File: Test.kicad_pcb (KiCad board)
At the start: 4 copper layers, 111.8 x 100.3 mm, 41 parts, among them P1 CONN_01X12, P10 CONN_01X12, P10a1 CONN_01X10, P11 CONN_01X03, P12 CONN_01X04, P13 CONN_02X04, P14 CONN_02X03, P15 CONN_02X05, P16 CONN_01X05, P17 CONN_01X01, P18 CONN_01X02, P19 CONN_01X08, P1a1 CONN_01X10, P2 CONN_01X12, P20 CONN_01X05, P21 CONN_01X05, P22 CONN_01X04, P23 CONN_01X04, P24 CONN_01X03, P25 CONN_01X10, P26 CONN_01X10, P27 CONN_01X10, P28 CONN_01X10, P2a1 CONN_01X10, P2a2 CONN_01X03, P2a3 CONN_01X03, P3 CONN_01X03, P4 CONN_01X24, P5 CONN_01X24, P6 CONN_01X03, P7 CONN_01X24, P8 CONN_01X24, P9 CONN_01X12, P9a1 CONN_01X10, SW1 SW_PUSH_SMALL_H, SW2 SW_PUSH_SMALL_H

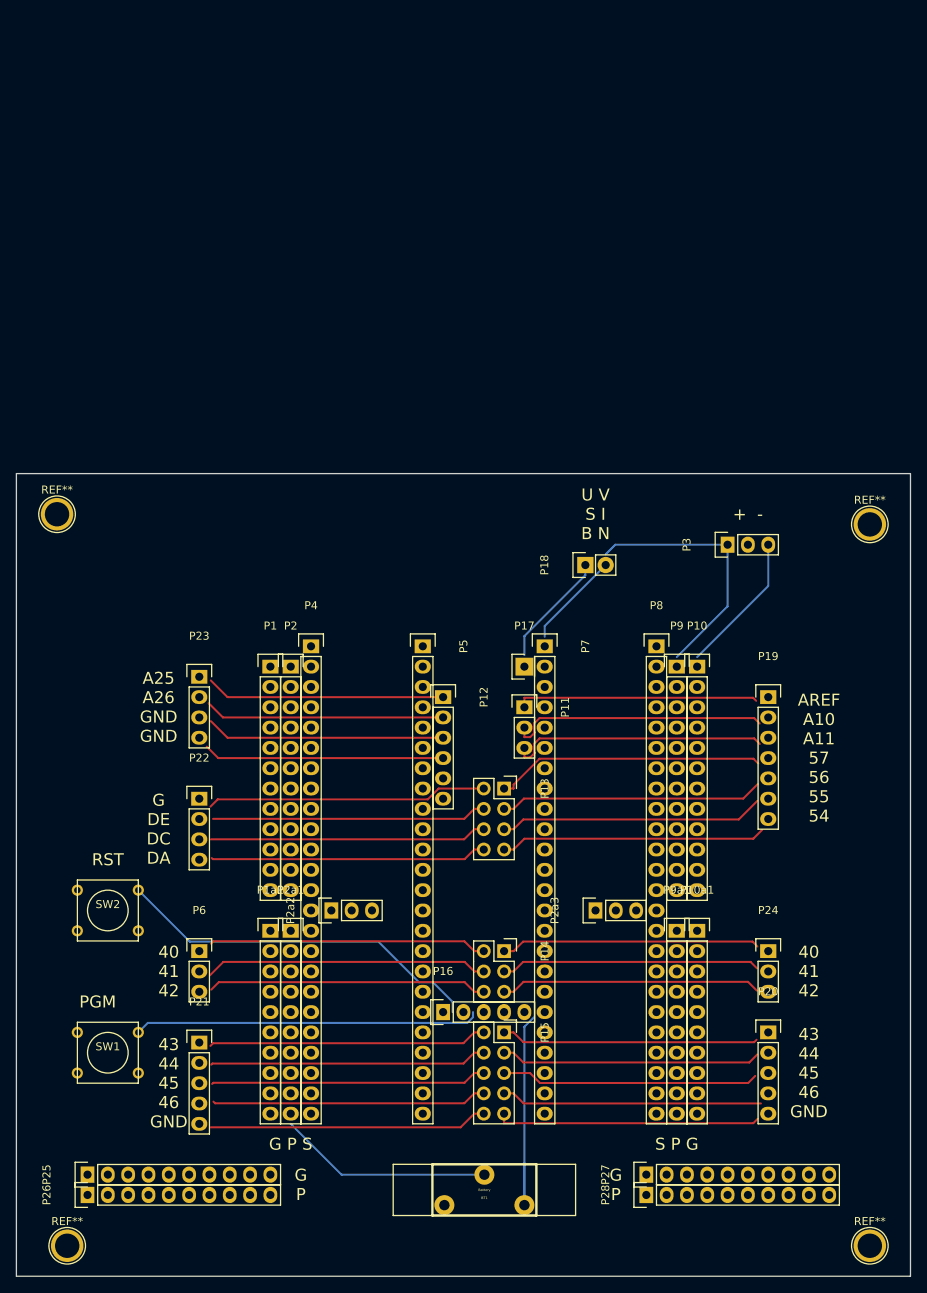
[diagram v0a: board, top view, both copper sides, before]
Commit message: Version 2
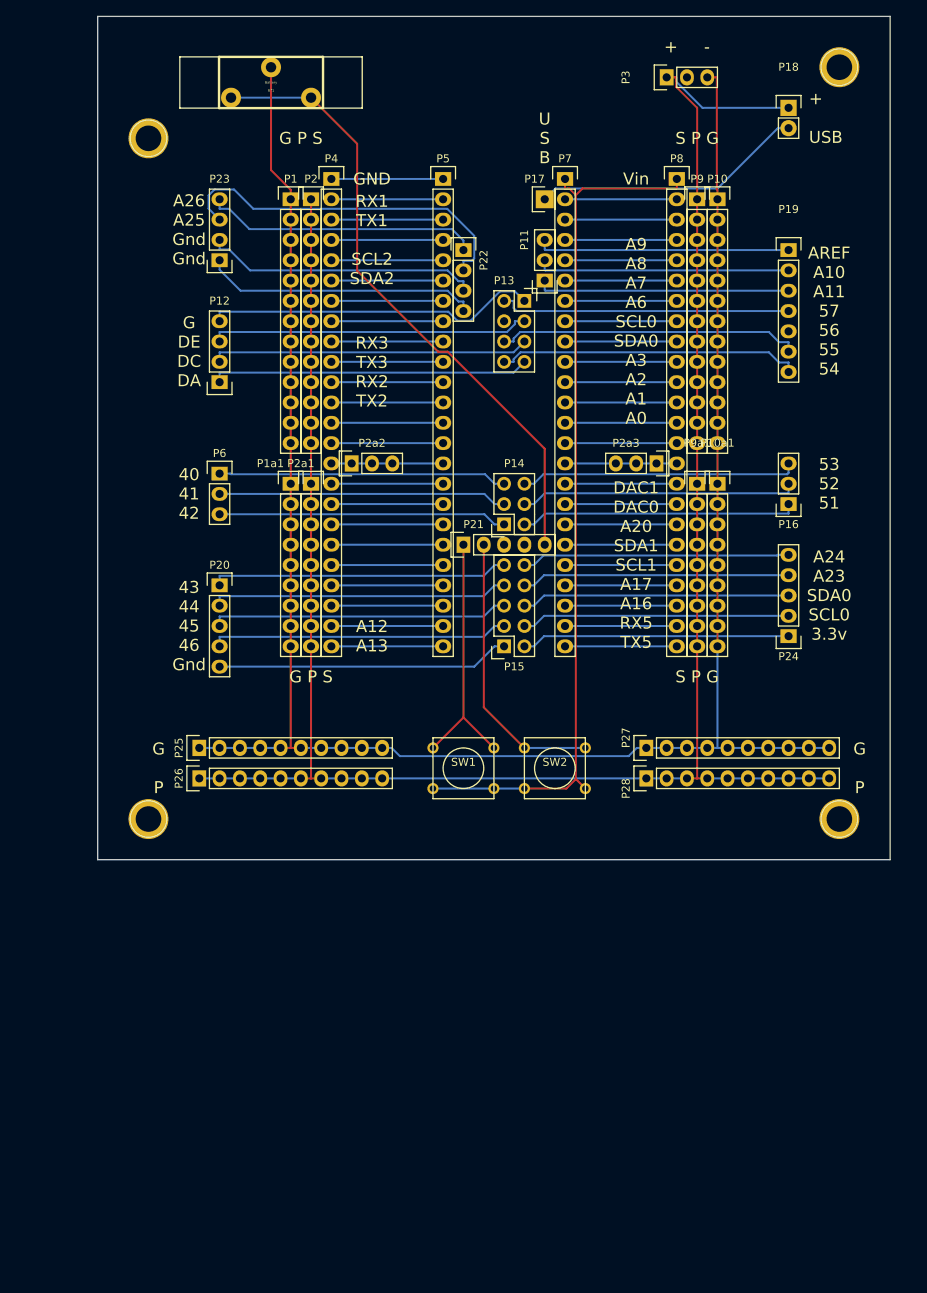
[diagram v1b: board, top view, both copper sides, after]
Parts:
- removed the REF** at (57.1, 184.2)
- removed the REF** at (157.5, 184.2)
- removed the REF** at (157.5, 94.0)
- removed the REF** at (55.9, 92.7)
- added REF**: 1pin, Connect:1pin, F.Cu at (153.7, 36.8)
- added REF**: 1pin, Connect:1pin, F.Cu at (67.3, 45.7)
- added REF**: 1pin, Connect:1pin, F.Cu at (67.3, 130.8)
- added REF**: 1pin, Connect:1pin, F.Cu at (153.7, 130.8)
- P1, P10, P2, P9: value CONN_01X12 -> CONN_01X13; footprint Pin_Headers:Pin_Header_Straight_1x12 -> Pin_Headers:Pin_Header_Straight_1x13
- P10a1: footprint Pin_Headers:Pin_Header_Straight_1x10 -> Pin_Headers:Pin_Header_Straight_1x09
- P12: footprint Socket_Strips:Socket_Strip_Straight_1x06 -> Pin_Headers:Pin_Header_Straight_1x04
- P16: value CONN_01X05 -> CONN_01X03; footprint Socket_Strips:Socket_Strip_Straight_1x05 -> Pin_Headers:Pin_Header_Straight_1x03
- P1a1, P2a1, P9a1: value CONN_01X10 -> CONN_01X09; footprint Pin_Headers:Pin_Header_Straight_1x10 -> Pin_Headers:Pin_Header_Straight_1x09
- P21: footprint Pin_Headers:Pin_Header_Straight_1x05 -> Socket_Strips:Socket_Strip_Straight_1x05
- P22: footprint Pin_Headers:Pin_Header_Straight_1x04 -> Socket_Strips:Socket_Strip_Straight_1x04
- P24: value CONN_01X03 -> CONN_01X05; footprint Pin_Headers:Pin_Header_Straight_1x03 -> Pin_Headers:Pin_Header_Straight_1x05
- moved BT1 141.0 mm to (82.6, 38.7)
- moved P20 88.5 mm to (76.2, 101.6)
- moved P16 76.8 mm to (147.3, 91.4), turned to 180 degrees
- moved P22 76.1 mm to (106.7, 59.7), turned to 270 degrees
- moved P21 70.4 mm to (106.7, 96.5)
- moved P18 62.5 mm to (147.3, 41.9), turned to 0 degrees
- moved P13 61.0 mm to (114.3, 66.0)
- moved P6 59.7 mm to (76.2, 87.6)
- moved P3 58.9 mm to (132.1, 38.1)
- moved SW2 58.6 mm to (118.1, 124.5)
- moved P1 58.5 mm to (85.1, 53.3)
- moved P10 58.5 mm to (138.4, 53.3)
- moved P17 58.5 mm to (116.8, 53.3)
- moved P2 58.5 mm to (87.6, 53.3)
- moved P4 58.5 mm to (90.2, 50.8)
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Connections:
- P1 pad 1: Net-(P1-Pad1) -> Net-(BT1-Pad2)
- P1 pad 10: Net-(P1-Pad1) -> Net-(BT1-Pad2)
- P1 pad 11: Net-(P1-Pad1) -> Net-(BT1-Pad2)
- P1 pad 12: Net-(P1-Pad1) -> Net-(BT1-Pad2)
- P1 pad 2: Net-(P1-Pad1) -> Net-(BT1-Pad2)
- P1 pad 3: Net-(P1-Pad1) -> Net-(BT1-Pad2)
- P1 pad 4: Net-(P1-Pad1) -> Net-(BT1-Pad2)
- P1 pad 5: Net-(P1-Pad1) -> Net-(BT1-Pad2)
- P1 pad 6: Net-(P1-Pad1) -> Net-(BT1-Pad2)
- P1 pad 7: Net-(P1-Pad1) -> Net-(BT1-Pad2)
- P1 pad 8: Net-(P1-Pad1) -> Net-(BT1-Pad2)
- P1 pad 9: Net-(P1-Pad1) -> Net-(BT1-Pad2)
- P10 pad 1: Net-(P10-Pad1) -> Net-(BT1-Pad2)
- P10 pad 10: Net-(P10-Pad1) -> Net-(BT1-Pad2)
- P10 pad 11: Net-(P10-Pad1) -> Net-(BT1-Pad2)
- P10 pad 12: Net-(P10-Pad1) -> Net-(BT1-Pad2)
- P10 pad 2: Net-(P10-Pad1) -> Net-(BT1-Pad2)
- P10 pad 3: Net-(P10-Pad1) -> Net-(BT1-Pad2)
- P10 pad 4: Net-(P10-Pad1) -> Net-(BT1-Pad2)
- P10 pad 5: Net-(P10-Pad1) -> Net-(BT1-Pad2)
- P10 pad 6: Net-(P10-Pad1) -> Net-(BT1-Pad2)
- P10 pad 7: Net-(P10-Pad1) -> Net-(BT1-Pad2)
- P10 pad 8: Net-(P10-Pad1) -> Net-(BT1-Pad2)
- P10 pad 9: Net-(P10-Pad1) -> Net-(BT1-Pad2)
- P10a1 pad 1: Net-(P10a1-Pad1) -> Net-(BT1-Pad2)
- P10a1 pad 2: Net-(P10a1-Pad1) -> Net-(BT1-Pad2)
- P10a1 pad 3: Net-(P10a1-Pad1) -> Net-(BT1-Pad2)
- P10a1 pad 4: Net-(P10a1-Pad1) -> Net-(BT1-Pad2)
- P10a1 pad 5: Net-(P10a1-Pad1) -> Net-(BT1-Pad2)
- P10a1 pad 6: Net-(P10a1-Pad1) -> Net-(BT1-Pad2)
- P10a1 pad 7: Net-(P10a1-Pad1) -> Net-(BT1-Pad2)
- P10a1 pad 8: Net-(P10a1-Pad1) -> Net-(BT1-Pad2)
- P10a1 pad 9: Net-(P10a1-Pad1) -> Net-(BT1-Pad2)
- P13 pad 1: Net-(P13-Pad1) -> Net-(P12-Pad4)
- P13 pad 3: Net-(P13-Pad3) -> Net-(P12-Pad3)
- P13 pad 5: Net-(P13-Pad5) -> Net-(P12-Pad2)
- P13 pad 7: Net-(P13-Pad7) -> Net-(P12-Pad1)
- P16 pad 1: Net-(P16-Pad1) -> Net-(P14-Pad2)
- P16 pad 2: Net-(P16-Pad2) -> Net-(P14-Pad4)
- P16 pad 3: Net-(P16-Pad3) -> Net-(P14-Pad6)
- P18 pad 2: Net-(P18-Pad2) -> Net-(P17-Pad1)
- P19 pad 1: Net-(P19-Pad1) -> Net-(P11-Pad3)
- P19 pad 2: Net-(P19-Pad2) -> Net-(P11-Pad2)
- P19 pad 3: Net-(P19-Pad3) -> Net-(P11-Pad1)
- P19 pad 4: Net-(P19-Pad4) -> Net-(P13-Pad2)
- P19 pad 6: Net-(P19-Pad6) -> Net-(P13-Pad6)
- P19 pad 7: Net-(P19-Pad7) -> Net-(P13-Pad8)
- P1a1 pad 1: Net-(P1a1-Pad1) -> Net-(BT1-Pad2)
- P1a1 pad 2: Net-(P1a1-Pad1) -> Net-(BT1-Pad2)
- P1a1 pad 3: Net-(P1a1-Pad1) -> Net-(BT1-Pad2)
- P1a1 pad 4: Net-(P1a1-Pad1) -> Net-(BT1-Pad2)
- P1a1 pad 5: Net-(P1a1-Pad1) -> Net-(BT1-Pad2)
- P1a1 pad 6: Net-(P1a1-Pad1) -> Net-(BT1-Pad2)
- P1a1 pad 7: Net-(P1a1-Pad1) -> Net-(BT1-Pad2)
- P1a1 pad 8: Net-(P1a1-Pad1) -> Net-(BT1-Pad2)
- P1a1 pad 9: Net-(P1a1-Pad1) -> Net-(BT1-Pad2)
- P2 pad 1: Net-(P2-Pad1) -> Net-(P18-Pad1)
- P2 pad 10: Net-(P2-Pad1) -> Net-(P18-Pad1)
- P2 pad 11: Net-(P2-Pad1) -> Net-(P18-Pad1)
- P2 pad 12: Net-(P2-Pad1) -> Net-(P18-Pad1)
- P2 pad 2: Net-(P2-Pad1) -> Net-(P18-Pad1)
- P2 pad 3: Net-(P2-Pad1) -> Net-(P18-Pad1)
- P2 pad 4: Net-(P2-Pad1) -> Net-(P18-Pad1)
- P2 pad 5: Net-(P2-Pad1) -> Net-(P18-Pad1)
- P2 pad 6: Net-(P2-Pad1) -> Net-(P18-Pad1)
- P2 pad 7: Net-(P2-Pad1) -> Net-(P18-Pad1)
- P2 pad 8: Net-(P2-Pad1) -> Net-(P18-Pad1)
- P2 pad 9: Net-(P2-Pad1) -> Net-(P18-Pad1)
- P20 pad 1: Net-(P20-Pad1) -> Net-(P15-Pad9)
- P20 pad 2: Net-(P20-Pad2) -> Net-(P15-Pad7)
- P20 pad 3: Net-(P20-Pad3) -> Net-(P15-Pad5)
- P20 pad 4: Net-(P20-Pad4) -> Net-(P15-Pad3)
- P20 pad 5: Net-(P20-Pad5) -> Net-(P15-Pad1)
- P21 pad 5: Net-(P21-Pad5) -> Net-(BT1-Pad1)
- P23 pad 1: Net-(P23-Pad1) -> Net-(P22-Pad4)
- P23 pad 2: Net-(P23-Pad2) -> Net-(P22-Pad3)
- P23 pad 3: Net-(P23-Pad3) -> Net-(P22-Pad2)
- P23 pad 4: Net-(P23-Pad4) -> Net-(P22-Pad1)
- P24 pad 1: Net-(P24-Pad1) -> Net-(P15-Pad2)
- P24 pad 2: Net-(P24-Pad2) -> Net-(P15-Pad4)
- P24 pad 3: Net-(P24-Pad3) -> Net-(P15-Pad6)
- P25 pad 1: Net-(P25-Pad1) -> Net-(BT1-Pad2)
- P25 pad 10: Net-(P25-Pad1) -> Net-(BT1-Pad2)
- P25 pad 2: Net-(P25-Pad1) -> Net-(BT1-Pad2)
- P25 pad 3: Net-(P25-Pad1) -> Net-(BT1-Pad2)
- P25 pad 4: Net-(P25-Pad1) -> Net-(BT1-Pad2)
- P25 pad 5: Net-(P25-Pad1) -> Net-(BT1-Pad2)
- P25 pad 6: Net-(P25-Pad1) -> Net-(BT1-Pad2)
- P25 pad 7: Net-(P25-Pad1) -> Net-(BT1-Pad2)
- P25 pad 8: Net-(P25-Pad1) -> Net-(BT1-Pad2)
- P25 pad 9: Net-(P25-Pad1) -> Net-(BT1-Pad2)
- P26 pad 1: Net-(P26-Pad1) -> Net-(P18-Pad1)
- P26 pad 10: Net-(P26-Pad1) -> Net-(P18-Pad1)
- P26 pad 2: Net-(P26-Pad1) -> Net-(P18-Pad1)
- P26 pad 3: Net-(P26-Pad1) -> Net-(P18-Pad1)
- P26 pad 4: Net-(P26-Pad1) -> Net-(P18-Pad1)
- P26 pad 5: Net-(P26-Pad1) -> Net-(P18-Pad1)
- P26 pad 6: Net-(P26-Pad1) -> Net-(P18-Pad1)
- P26 pad 7: Net-(P26-Pad1) -> Net-(P18-Pad1)
- P26 pad 8: Net-(P26-Pad1) -> Net-(P18-Pad1)
- P26 pad 9: Net-(P26-Pad1) -> Net-(P18-Pad1)
- P27 pad 1: Net-(P27-Pad1) -> Net-(BT1-Pad2)
- P27 pad 10: Net-(P27-Pad1) -> Net-(BT1-Pad2)
- P27 pad 2: Net-(P27-Pad1) -> Net-(BT1-Pad2)
- P27 pad 3: Net-(P27-Pad1) -> Net-(BT1-Pad2)
- P27 pad 4: Net-(P27-Pad1) -> Net-(BT1-Pad2)
- P27 pad 5: Net-(P27-Pad1) -> Net-(BT1-Pad2)
- P27 pad 6: Net-(P27-Pad1) -> Net-(BT1-Pad2)
- P27 pad 7: Net-(P27-Pad1) -> Net-(BT1-Pad2)
- P27 pad 8: Net-(P27-Pad1) -> Net-(BT1-Pad2)
- P27 pad 9: Net-(P27-Pad1) -> Net-(BT1-Pad2)
- P28 pad 1: Net-(P28-Pad1) -> Net-(P18-Pad1)
- P28 pad 10: Net-(P28-Pad1) -> Net-(P18-Pad1)
- P28 pad 2: Net-(P28-Pad1) -> Net-(P18-Pad1)
- P28 pad 3: Net-(P28-Pad1) -> Net-(P18-Pad1)
- P28 pad 4: Net-(P28-Pad1) -> Net-(P18-Pad1)
- P28 pad 5: Net-(P28-Pad1) -> Net-(P18-Pad1)
- P28 pad 6: Net-(P28-Pad1) -> Net-(P18-Pad1)
- P28 pad 7: Net-(P28-Pad1) -> Net-(P18-Pad1)
- P28 pad 8: Net-(P28-Pad1) -> Net-(P18-Pad1)
- P28 pad 9: Net-(P28-Pad1) -> Net-(P18-Pad1)
- P2a1 pad 1: Net-(P2a1-Pad1) -> Net-(P18-Pad1)
- P2a1 pad 2: Net-(P2a1-Pad1) -> Net-(P18-Pad1)
- P2a1 pad 3: Net-(P2a1-Pad1) -> Net-(P18-Pad1)
- P2a1 pad 4: Net-(P2a1-Pad1) -> Net-(P18-Pad1)
- P2a1 pad 5: Net-(P2a1-Pad1) -> Net-(P18-Pad1)
- P2a1 pad 6: Net-(P2a1-Pad1) -> Net-(P18-Pad1)
- P2a1 pad 7: Net-(P2a1-Pad1) -> Net-(P18-Pad1)
- P2a1 pad 8: Net-(P2a1-Pad1) -> Net-(P18-Pad1)
- P2a1 pad 9: Net-(P2a1-Pad1) -> Net-(P18-Pad1)
- P3 pad 1: Net-(P3-Pad1) -> Net-(P18-Pad1)
- P3 pad 3: GND -> Net-(BT1-Pad2)
- P4 pad 14: Net-(P2a2-Pad1) -> Net-(P4-Pad14)
- P4 pad 15: Net-(P4-Pad15) -> Net-(P2a2-Pad1)
- P5 pad 14: Net-(P2a2-Pad1) -> Net-(P4-Pad14)
- P5 pad 15: Net-(P4-Pad15) -> Net-(P2a2-Pad1)
- P6 pad 1: Net-(P6-Pad1) -> Net-(P14-Pad5)
- P6 pad 2: Net-(P6-Pad2) -> Net-(P14-Pad3)
- P6 pad 3: Net-(P6-Pad3) -> Net-(P14-Pad1)
- P7 pad 14: Net-(P2a3-Pad1) -> Net-(P7-Pad14)
- P7 pad 15: Net-(P7-Pad15) -> Net-(P2a3-Pad1)
- P8 pad 14: Net-(P2a3-Pad1) -> Net-(P7-Pad14)
- P8 pad 15: Net-(P7-Pad15) -> Net-(P2a3-Pad1)
- P9 pad 1: Net-(P9-Pad1) -> Net-(P18-Pad1)
- P9 pad 10: Net-(P9-Pad1) -> Net-(P18-Pad1)
- P9 pad 11: Net-(P9-Pad1) -> Net-(P18-Pad1)
- P9 pad 12: Net-(P9-Pad1) -> Net-(P18-Pad1)
- P9 pad 2: Net-(P9-Pad1) -> Net-(P18-Pad1)
- P9 pad 3: Net-(P9-Pad1) -> Net-(P18-Pad1)
- P9 pad 4: Net-(P9-Pad1) -> Net-(P18-Pad1)
- P9 pad 5: Net-(P9-Pad1) -> Net-(P18-Pad1)
- P9 pad 6: Net-(P9-Pad1) -> Net-(P18-Pad1)
- P9 pad 7: Net-(P9-Pad1) -> Net-(P18-Pad1)
- P9 pad 8: Net-(P9-Pad1) -> Net-(P18-Pad1)
- P9 pad 9: Net-(P9-Pad1) -> Net-(P18-Pad1)
- P9a1 pad 1: Net-(P9a1-Pad1) -> Net-(P18-Pad1)
- P9a1 pad 2: Net-(P9a1-Pad1) -> Net-(P18-Pad1)
- P9a1 pad 3: Net-(P9a1-Pad1) -> Net-(P18-Pad1)
- P9a1 pad 4: Net-(P9a1-Pad1) -> Net-(P18-Pad1)
- P9a1 pad 5: Net-(P9a1-Pad1) -> Net-(P18-Pad1)
- P9a1 pad 6: Net-(P9a1-Pad1) -> Net-(P18-Pad1)
- P9a1 pad 7: Net-(P9a1-Pad1) -> Net-(P18-Pad1)
- P9a1 pad 8: Net-(P9a1-Pad1) -> Net-(P18-Pad1)
- P9a1 pad 9: Net-(P9a1-Pad1) -> Net-(P18-Pad1)
- SW1 pad 1: Net-(SW1-Pad1) -> Net-(P21-Pad1)
- SW1 pad 2: Net-(SW1-Pad2) -> Net-(P7-Pad1)
- SW2 pad 1: Net-(SW2-Pad1) -> Net-(P21-Pad2)
- SW2 pad 2: Net-(SW2-Pad2) -> Net-(P7-Pad1)
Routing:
- net Net-(P18-Pad1): track 14.4 -> 258.2 mm
- net Net-(BT1-Pad2): track 26.8 -> 250.7 mm
- net Net-(P7-Pad1): track 14.0 -> 110.1 mm
- net Net-(P1-Pad1): track 85.6 -> 0.00 mm
- net Net-(P2-Pad1): track 81.0 -> 0.00 mm
- net Net-(SW2-Pad1): track 54.0 -> 0.00 mm
- net Net-(SW1-Pad2): track 52.4 -> 0.00 mm
- net Net-(SW1-Pad1): track 50.9 -> 0.00 mm
- net Net-(P22-Pad2): track 0.00 -> 45.0 mm
- net Net-(BT1-Pad1): track 39.2 -> 78.7 mm
- net Net-(P21-Pad2): track 0.00 -> 35.1 mm
- net Net-(P22-Pad4): track 0.00 -> 34.5 mm
- net Net-(P22-Pad3): track 0.00 -> 34.5 mm
- net Net-(P22-Pad1): track 0.00 -> 34.5 mm
- net Net-(P13-Pad4): track 34.4 -> 0.00 mm
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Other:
- board size 111.8 x 100.3 mm -> 99.1 x 105.4 mm
- copper layers 4 -> 2
- board text added: "+ USB"
- board text added: "43 44 45 46 Gnd"
- board text added: "53 52 51"
- board text added: "A12 A13"
- board text added: "A24 A23 SDA0 SCL0 3.3v"
- board text added: "A26 A25 Gnd Gnd"
- board text added: "A9 A8 A7 A6 SCL0 SDA0 A3 A2 A1 A0"
- board text added: "DAC1 DAC0 A20 SDA1 SCL1 A17 A16 RX5 TX5"
- board text added: "GND"
- board text added: "RX1 TX1 SCL2 SDA2"
- board text added: "RX3 TX3 RX2 TX2"
- board text added: "U S B"
- board text added: "Vin"
- board text removed: "43 44 45 46 GND"
- board text removed: "A25 A26 GND GND"
- board text removed: "PGM"
- board text removed: "RST"
- board text removed: "U V S I B N"
